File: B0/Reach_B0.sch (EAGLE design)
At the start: 239 parts, among them IC1 TMC2100-LA, IC10 74AHC1G126DCK, IC11 74AHC1G126DCK, IC18 74AHC1G126DCK, IC2 TMC2100-LA, IC3 74AHC1G126DCK, IC4 74AHC1G126DCK, IC5 74AHC1G126DCK, IC6 74AHC1G126DCK, IC7 74AHC1G126DCK, IC8 TMC2100-LA, IC9 74AHC1G126DCK, P8 F-2X23-, P9 F-2X23-, Q2 AON6758, Q3 AON6758, U1 SN74AHC595PW, U10 RT8268, U11 PCA9685PW, U18 CAT24C256, U2 SN74AHC595PW, U3 MCP9600, U4 MCP9600, U5 MCP9600, U6 MCP9600, U7 SN74AHC595PW, X1 22-05-7028-02, X11 22-05-7028-02, X14 22-05-7048-04, X2 MSTBA4, X21 MSTBA2, X3 MSTBA2, X4 22-05-7028-02, X5 22-05-7028-02, X6 22-05-7048-04, X7 22-05-7028-02, X8 22-05-7048-04, X9 22-05-7028-02

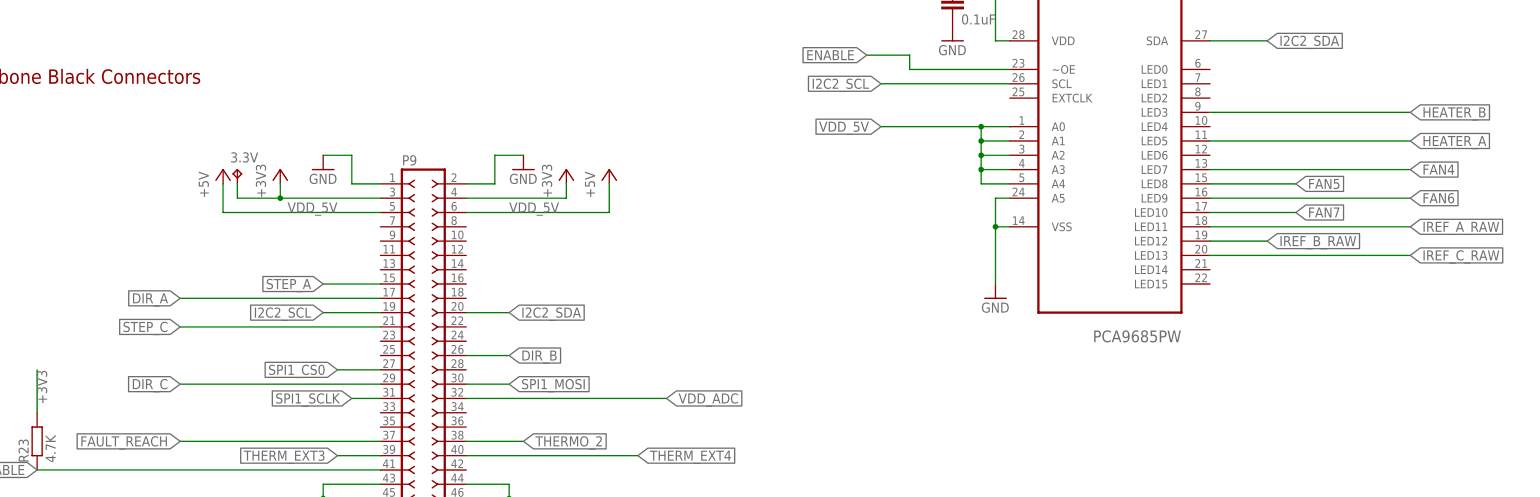
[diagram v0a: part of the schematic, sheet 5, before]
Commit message: Add files via upload
Changed pinout to make layout simpler
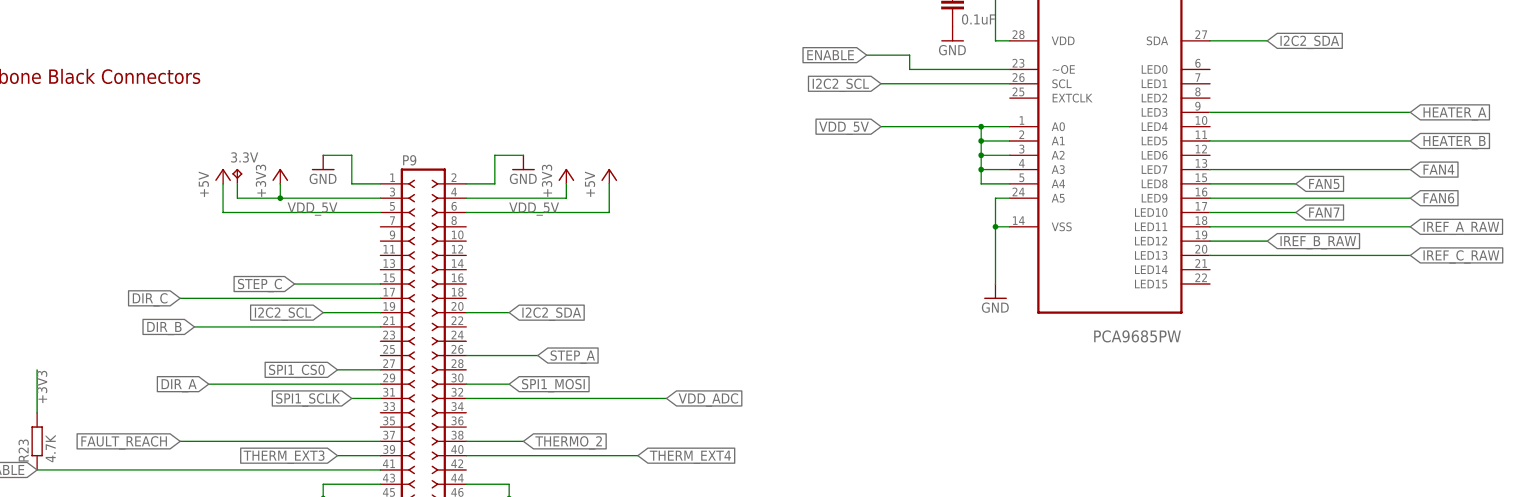
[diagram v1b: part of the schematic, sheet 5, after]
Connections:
- net DIR_A: now also P9.29; no longer P9.17
- net DIR_B: now also P9.21; no longer P9.26
- net DIR_C: now also P9.17; no longer P9.29
- net HEATER_A: now also U11.LED3; no longer U11.LED5
- net HEATER_B: now also U11.LED5; no longer U11.LED3
- net SPI1_CS0: now also P9.27
- net STEP_A: now also P9.26; no longer P9.15
- net STEP_C: now also P9.15; no longer P9.21
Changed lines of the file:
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@@
 <?xml version="1.0" encoding="utf-8"?>
 <!DOCTYPE eagle SYSTEM "eagle.dtd">
-<eagle version="8.1.0">
+<eagle version="8.1.1">
 <drawing>
 <settings>
@@
 <setting verticaltext="up"/>
 </settings>
-<grid distance="0.1" unitdist="inch" unit="inch" style="lines" multiple="1" display="no" altdistance="0.01" altunitdist="inch" altunit="inch"/>
+<grid distance="0.1" unitdist="inch" unit="mm" style="lines" multiple="1" display="no" altdistance="0.01" altunitdist="inch" altunit="inch"/>
 <layers>
 <layer number="1" name="Top" color="4" fill="1" visible="no" active="no"/>
@@
 <segment>
 <label x="157.48" y="53.34" size="1.778" layer="95" rot="R180" xref="yes"/>
-<wire x1="165.1" y1="53.34" x2="157.48" y2="53.34" width="0.1524" layer="91"/>
+<pinref part="P9" gate="G$1" pin="27"/>
+<wire x1="157.48" y1="53.34" x2="165.1" y2="53.34" width="0.1524" layer="91"/>
 </segment>
 </net>
@@
 <net name="DIR_B" class="0">
 <segment>
-<pinref part="P9" gate="G$1" pin="26"/>
-<wire x1="180.34" y1="55.88" x2="187.96" y2="55.88" width="0.1524" layer="91"/>
-<label x="187.96" y="55.88" size="1.778" layer="95" xref="yes"/>
+<label x="132.08" y="60.96" size="1.778" layer="95" rot="R180" xref="yes"/>
+<pinref part="P9" gate="G$1" pin="21"/>
+<wire x1="165.1" y1="60.96" x2="132.08" y2="60.96" width="0.1524" layer="91"/>
 </segment>
 </net>
@@
 <net name="STEP_A" class="0">
 <segment>
-<pinref part="P9" gate="G$1" pin="15"/>
-<label x="154.94" y="68.58" size="1.778" layer="95" rot="R180" xref="yes"/>
-<wire x1="165.1" y1="68.58" x2="154.94" y2="68.58" width="0.1524" layer="91"/>
+<label x="193.04" y="55.88" size="1.778" layer="95" xref="yes"/>
+<pinref part="P9" gate="G$1" pin="26"/>
+<wire x1="180.34" y1="55.88" x2="193.04" y2="55.88" width="0.1524" layer="91"/>
 </segment>
 </net>
 <net name="DIR_A" class="0">
 <segment>
-<pinref part="P9" gate="G$1" pin="17"/>
-<label x="129.54" y="66.04" size="1.778" layer="95" rot="R180" xref="yes"/>
-<wire x1="165.1" y1="66.04" x2="129.54" y2="66.04" width="0.1524" layer="91"/>
+<label x="134.62" y="50.8" size="1.778" layer="95" rot="R180" xref="yes"/>
+<pinref part="P9" gate="G$1" pin="29"/>
+<wire x1="134.62" y1="50.8" x2="165.1" y2="50.8" width="0.1524" layer="91"/>
 </segment>
 </net>
@@
 <net name="DIR_C" class="0">
 <segment>
-<pinref part="P9" gate="G$1" pin="29"/>
-<wire x1="165.1" y1="50.8" x2="129.54" y2="50.8" width="0.1524" layer="91"/>
-<label x="129.54" y="50.8" size="1.778" layer="95" rot="R180" xref="yes"/>
+<label x="129.54" y="66.04" size="1.778" layer="95" rot="R180" xref="yes"/>
+<pinref part="P9" gate="G$1" pin="17"/>
+<wire x1="165.1" y1="66.04" x2="129.54" y2="66.04" width="0.1524" layer="91"/>
 </segment>
 </net>
 <net name="STEP_C" class="0">
 <segment>
-<pinref part="P9" gate="G$1" pin="21"/>
-<wire x1="165.1" y1="60.96" x2="129.54" y2="60.96" width="0.1524" layer="91"/>
-<label x="129.54" y="60.96" size="1.778" layer="95" rot="R180" xref="yes"/>
+<label x="149.86" y="68.58" size="1.778" layer="95" rot="R180" xref="yes"/>
+<pinref part="P9" gate="G$1" pin="15"/>
+<wire x1="165.1" y1="68.58" x2="149.86" y2="68.58" width="0.1524" layer="91"/>
 </segment>
 </net>
@@
 <net name="HEATER_B" class="0">
 <segment>
-<pinref part="U11" gate="A" pin="LED3"/>
-<wire x1="312.42" y1="99.06" x2="347.98" y2="99.06" width="0.1524" layer="91"/>
-<label x="347.98" y="99.06" size="1.778" layer="95" xref="yes"/>
+<label x="347.98" y="93.98" size="1.778" layer="95" xref="yes"/>
+<wire x1="312.42" y1="93.98" x2="347.98" y2="93.98" width="0.1524" layer="91"/>
+<pinref part="U11" gate="A" pin="LED5"/>
 </segment>
 </net>
 <net name="HEATER_A" class="0">
 <segment>
-<pinref part="U11" gate="A" pin="LED5"/>
-<wire x1="312.42" y1="93.98" x2="347.98" y2="93.98" width="0.1524" layer="91"/>
-<label x="347.98" y="93.98" size="1.778" layer="95" xref="yes"/>
+<label x="347.98" y="99.06" size="1.778" layer="95" xref="yes"/>
+<pinref part="U11" gate="A" pin="LED3"/>
+<wire x1="347.98" y1="99.06" x2="312.42" y2="99.06" width="0.1524" layer="91"/>
 </segment>
 </net>
